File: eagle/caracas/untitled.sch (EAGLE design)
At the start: 12 parts, among them IC1 ICM7555

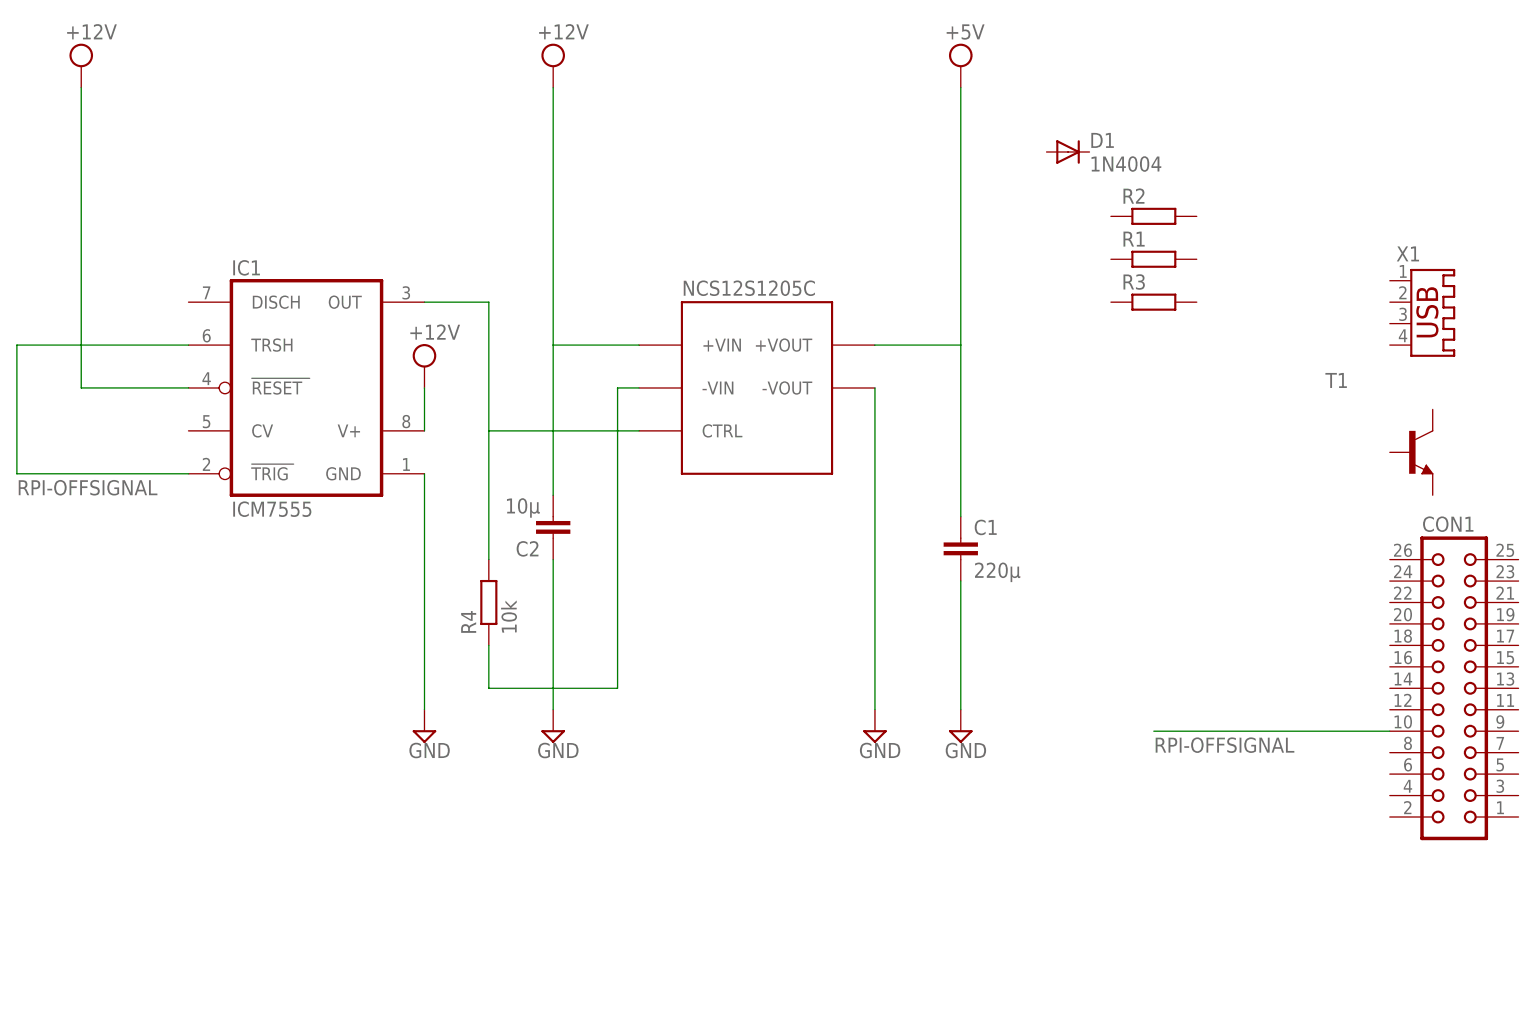
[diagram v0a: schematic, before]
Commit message: Update Eagle project.
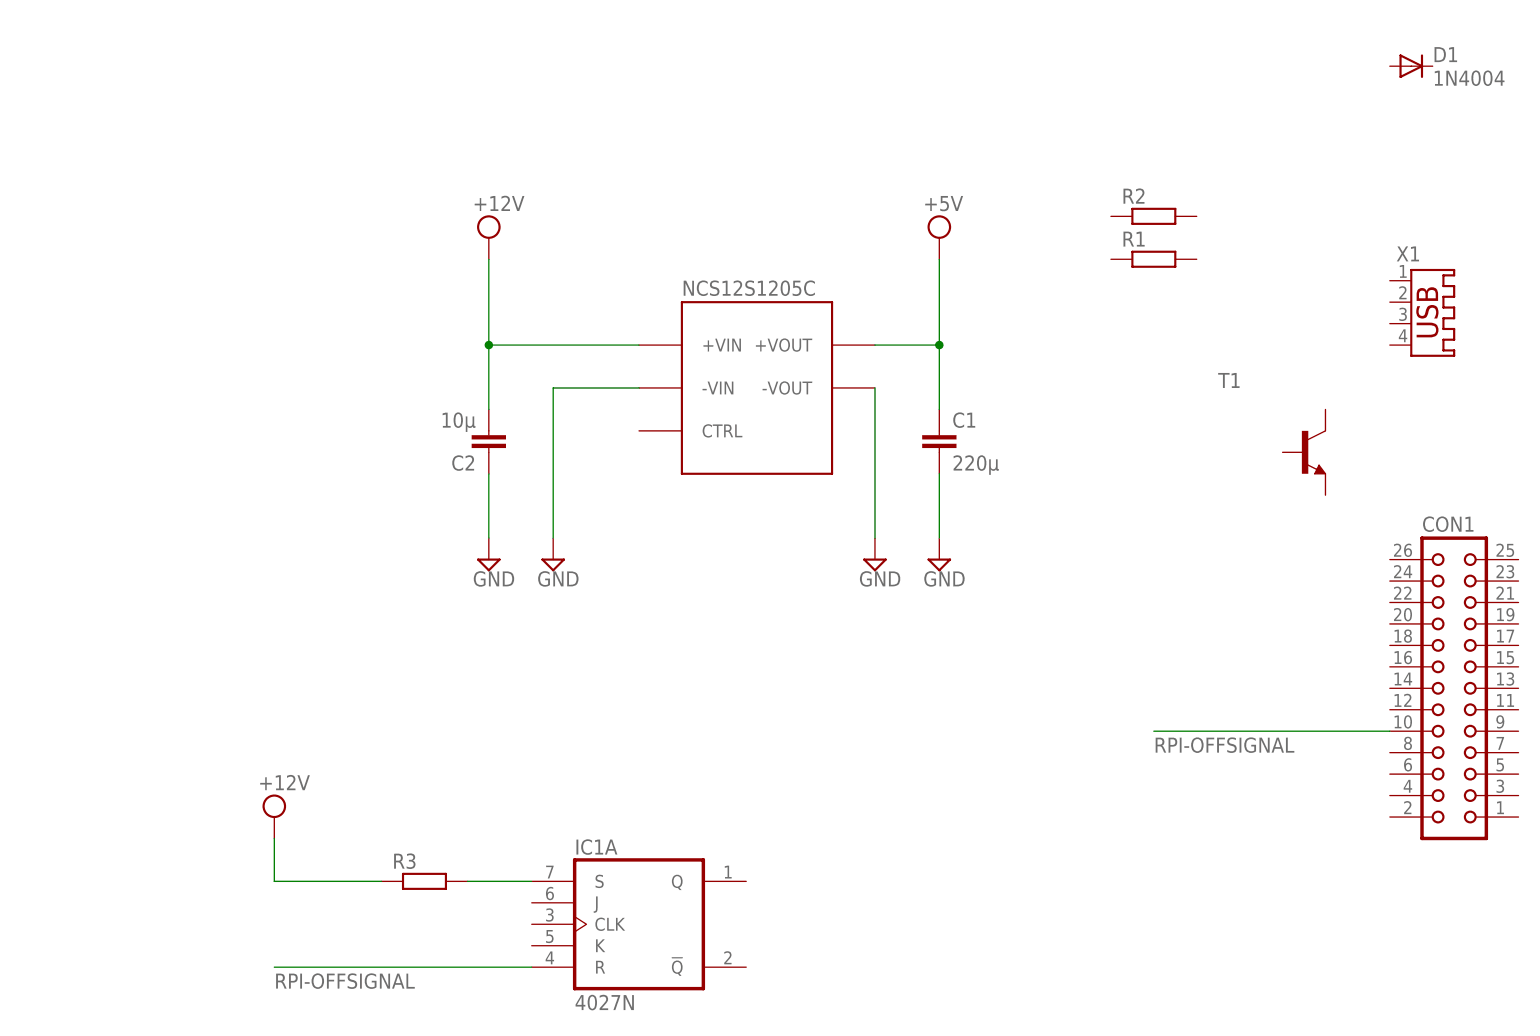
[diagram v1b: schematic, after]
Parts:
- removed R4: 10k, rcl:R-EU_0204/7
- IC1: value ICM7555 -> 4027N; device maxim:ICM7555 -> 40xx:4027N
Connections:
- removed net VCC: C1.1, C2.2, IC1.RESET, IC1.V+, U$1.+VIN, U$1.+VOUT
- new net +12V: C2.2, U$1.+VIN
- new net +12V_IGN: R3.1
- new net +5V: C1.1, U$1.+VOUT
- net GND: no longer IC1.GND, R4.1
- net N$1: now also IC1A.S, R3.2; no longer IC1.OUT, R4.2, U$1.CTRL
- net RPI-OFFSIGNAL: now also IC1A.R; no longer IC1.TRIG, IC1.TRSH
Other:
- moved on the sheet: C1, C2, D1, R3, T1
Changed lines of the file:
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@@
 <setting verticaltext="up"/>
 </settings>
-<grid distance="0.1" unitdist="inch" unit="inch" style="lines" multiple="1" display="yes" altdistance="0.01" altunitdist="inch" altunit="inch"/>
+<grid distance="0.1" unitdist="inch" unit="inch" style="lines" multiple="1" display="no" altdistance="0.01" altunitdist="inch" altunit="inch"/>
 <layers>
 <layer number="1" name="Top" color="4" fill="1" visible="no" active="no"/>
@@
 <part name="R2" library="rcl" deviceset="R-EU_" device="0207/10"/>
 <part name="R3" library="rcl" deviceset="R-EU_" device="0207/10"/>
-<part name="IC1" library="maxim" deviceset="ICM7555" device=""/>
 <part name="X1" library="con-yamaichi" deviceset="USB-A003" device=""/>
 <part name="CON1" library="con-harting" deviceset="CON26" device=""/>
@@
 <part name="D1" library="diode" deviceset="1N4004" device=""/>
 <part name="U$1" library="caracas" deviceset="NCS12S1205C" device=""/>
-<part name="R4" library="rcl" deviceset="R-EU_" device="0204/7" value="10k"/>
 <part name="SUPPLY1" library="supply2" deviceset="GND" device=""/>
 <part name="C1" library="rcl" deviceset="C-EU" device="025-024X044" value="220µ"/>
@@
 <part name="SUPPLY2" library="supply2" deviceset="GND" device=""/>
 <part name="SUPPLY3" library="supply2" deviceset="GND" device=""/>
-<part name="+12V" library="supply2" deviceset="VCC" device="" value="+12V"/>
 <part name="+5V" library="supply2" deviceset="VCC" device="" value="+5V"/>
+<part name="+12V2" library="supply2" deviceset="VCC" device="" value="+12V"/>
 <part name="SUPPLY4" library="supply2" deviceset="GND" device=""/>
-<part name="+12V1" library="supply2" deviceset="VCC" device="" value="+12V"/>
-<part name="+12V2" library="supply2" deviceset="VCC" device="" value="+12V"/>
+<part name="IC1" library="40xx" deviceset="4027" device="N"/>
+<part name="+12V_IGN" library="supply2" deviceset="VCC" device="" value="+12V"/>
 </parts>
 <sheets>
@@
 <instance part="R1" gate="G$1" x="106.68" y="73.66"/>
 <instance part="R2" gate="G$1" x="106.68" y="78.74"/>
-<instance part="R3" gate="G$1" x="106.68" y="68.58"/>
-<instance part="IC1" gate="G$1" x="7.62" y="58.42"/>
+<instance part="R3" gate="G$1" x="20.32" y="0"/>
 <instance part="X1" gate="G$1" x="139.7" y="66.04"/>
 <instance part="CON1" gate="A" x="142.24" y="22.86"/>
-<instance part="T1" gate="G$1" x="137.16" y="50.8"/>
-<instance part="D1" gate="1" x="96.52" y="86.36"/>
+<instance part="T1" gate="G$1" x="124.46" y="50.8"/>
+<instance part="D1" gate="1" x="137.16" y="96.52"/>
 <instance part="U$1" gate="G$1" x="58.42" y="58.42"/>
-<instance part="R4" gate="G$1" x="27.94" y="33.02" rot="R90"/>
-<instance part="SUPPLY1" gate="GND" x="35.56" y="17.78"/>
-<instance part="C1" gate="G$1" x="83.82" y="40.64"/>
-<instance part="C2" gate="G$1" x="35.56" y="40.64" rot="R180"/>
-<instance part="SUPPLY2" gate="GND" x="73.66" y="17.78"/>
-<instance part="SUPPLY3" gate="GND" x="83.82" y="17.78"/>
-<instance part="+12V" gate="G$1" x="-20.32" y="96.52"/>
-<instance part="+5V" gate="G$1" x="83.82" y="96.52"/>
-<instance part="SUPPLY4" gate="GND" x="20.32" y="17.78"/>
-<instance part="+12V1" gate="G$1" x="20.32" y="60.96"/>
-<instance part="+12V2" gate="G$1" x="35.56" y="96.52"/>
+<instance part="SUPPLY1" gate="GND" x="27.94" y="38.1"/>
+<instance part="C1" gate="G$1" x="81.28" y="53.34"/>
+<instance part="C2" gate="G$1" x="27.94" y="50.8" rot="R180"/>
+<instance part="SUPPLY2" gate="GND" x="73.66" y="38.1"/>
+<instance part="SUPPLY3" gate="GND" x="81.28" y="38.1"/>
+<instance part="+5V" gate="G$1" x="81.28" y="76.2"/>
+<instance part="+12V2" gate="G$1" x="27.94" y="76.2"/>
+<instance part="SUPPLY4" gate="GND" x="35.56" y="38.1"/>
+<instance part="IC1" gate="A" x="45.72" y="-5.08"/>
+<instance part="+12V_IGN" gate="G$1" x="2.54" y="7.62"/>
 </instances>
 <busses>
 </busses>
 <nets>
-<net name="N$1" class="0">
-<segment>
-<pinref part="IC1" gate="G$1" pin="OUT"/>
-<wire x1="20.32" y1="68.58" x2="27.94" y2="68.58" width="0.1524" layer="91"/>
-<wire x1="27.94" y1="68.58" x2="27.94" y2="53.34" width="0.1524" layer="91"/>
-<pinref part="U$1" gate="G$1" pin="CTRL"/>
-<wire x1="27.94" y1="53.34" x2="45.72" y2="53.34" width="0.1524" layer="91"/>
-<wire x1="27.94" y1="53.34" x2="27.94" y2="38.1" width="0.1524" layer="91"/>
-<pinref part="R4" gate="G$1" pin="2"/>
-</segment>
-</net>
 <net name="GND" class="0">
 <segment>
 <pinref part="SUPPLY1" gate="GND" pin="GND"/>
-<pinref part="R4" gate="G$1" pin="1"/>
-<wire x1="35.56" y1="20.32" x2="35.56" y2="22.86" width="0.1524" layer="91"/>
-<pinref part="U$1" gate="G$1" pin="-VIN"/>
-<wire x1="35.56" y1="22.86" x2="27.94" y2="22.86" width="0.1524" layer="91"/>
-<wire x1="27.94" y1="22.86" x2="27.94" y2="27.94" width="0.1524" layer="91"/>
-<wire x1="45.72" y1="58.42" x2="43.18" y2="58.42" width="0.1524" layer="91"/>
-<wire x1="43.18" y1="58.42" x2="43.18" y2="22.86" width="0.1524" layer="91"/>
-<wire x1="43.18" y1="22.86" x2="35.56" y2="22.86" width="0.1524" layer="91"/>
 <pinref part="C2" gate="G$1" pin="1"/>
-<wire x1="35.56" y1="38.1" x2="35.56" y2="22.86" width="0.1524" layer="91"/>
+<wire x1="27.94" y1="48.26" x2="27.94" y2="40.64" width="0.1524" layer="91"/>
 </segment>
 <segment>
 <pinref part="U$1" gate="G$1" pin="-VOUT"/>
-<wire x1="73.66" y1="58.42" x2="73.66" y2="20.32" width="0.1524" layer="91"/>
+<wire x1="73.66" y1="58.42" x2="73.66" y2="40.64" width="0.1524" layer="91"/>
 <pinref part="SUPPLY2" gate="GND" pin="GND"/>
 </segment>
@@
 <pinref part="C1" gate="G$1" pin="2"/>
 <pinref part="SUPPLY3" gate="GND" pin="GND"/>
-<wire x1="83.82" y1="35.56" x2="83.82" y2="20.32" width="0.1524" layer="91"/>
+<wire x1="81.28" y1="48.26" x2="81.28" y2="40.64" width="0.1524" layer="91"/>
 </segment>
 <segment>
-<pinref part="IC1" gate="G$1" pin="GND"/>
-<wire x1="20.32" y1="48.26" x2="20.32" y2="20.32" width="0.1524" layer="91"/>
+<pinref part="U$1" gate="G$1" pin="-VIN"/>
+<wire x1="45.72" y1="58.42" x2="35.56" y2="58.42" width="0.1524" layer="91"/>
 <pinref part="SUPPLY4" gate="GND" pin="GND"/>
+<wire x1="35.56" y1="40.64" x2="35.56" y2="58.42" width="0.1524" layer="91"/>
 </segment>
 </net>
-<net name="VCC" class="0">
-<segment>
-<pinref part="+12V" gate="G$1" pin="VCC"/>
-<pinref part="IC1" gate="G$1" pin="RESET"/>
-<wire x1="-7.62" y1="58.42" x2="-20.32" y2="58.42" width="0.1524" layer="91"/>
-<wire x1="-20.32" y1="58.42" x2="-20.32" y2="93.98" width="0.1524" layer="91"/>
-</segment>
+<net name="+5V" class="0">
 <segment>
 <pinref part="C1" gate="G$1" pin="1"/>
-<wire x1="83.82" y1="43.18" x2="83.82" y2="63.5" width="0.1524" layer="91"/>
+<wire x1="81.28" y1="55.88" x2="81.28" y2="63.5" width="0.1524" layer="91"/>
 <pinref part="U$1" gate="G$1" pin="+VOUT"/>
-<wire x1="83.82" y1="63.5" x2="73.66" y2="63.5" width="0.1524" layer="91"/>
+<wire x1="81.28" y1="63.5" x2="73.66" y2="63.5" width="0.1524" layer="91"/>
 <pinref part="+5V" gate="G$1" pin="VCC"/>
-<wire x1="83.82" y1="93.98" x2="83.82" y2="63.5" width="0.1524" layer="91"/>
-</segment>
-<segment>
-<pinref part="IC1" gate="G$1" pin="V+"/>
-<pinref part="+12V1" gate="G$1" pin="VCC"/>
-<wire x1="20.32" y1="53.34" x2="20.32" y2="58.42" width="0.1524" layer="91"/>
-</segment>
-<segment>
-<pinref part="C2" gate="G$1" pin="2"/>
-<wire x1="35.56" y1="45.72" x2="35.56" y2="63.5" width="0.1524" layer="91"/>
-<pinref part="U$1" gate="G$1" pin="+VIN"/>
-<wire x1="35.56" y1="63.5" x2="45.72" y2="63.5" width="0.1524" layer="91"/>
-<pinref part="+12V2" gate="G$1" pin="VCC"/>
-<wire x1="35.56" y1="63.5" x2="35.56" y2="93.98" width="0.1524" layer="91"/>
+<wire x1="81.28" y1="73.66" x2="81.28" y2="63.5" width="0.1524" layer="91"/>
+<junction x="81.28" y="63.5"/>
 </segment>
 </net>
@@
 </segment>
 <segment>
-<pinref part="IC1" gate="G$1" pin="TRIG"/>
-<wire x1="-7.62" y1="48.26" x2="-27.94" y2="48.26" width="0.1524" layer="91"/>
-<label x="-27.94" y="45.72" size="1.778" layer="95"/>
-<pinref part="IC1" gate="G$1" pin="TRSH"/>
-<wire x1="-7.62" y1="63.5" x2="-27.94" y2="63.5" width="0.1524" layer="91"/>
-<wire x1="-27.94" y1="63.5" x2="-27.94" y2="48.26" width="0.1524" layer="91"/>
+<pinref part="IC1" gate="A" pin="R"/>
+<wire x1="33.02" y1="-10.16" x2="2.54" y2="-10.16" width="0.1524" layer="91"/>
+<label x="2.54" y="-12.7" size="1.778" layer="95"/>
 </segment>
 </net>
+<net name="N$1" class="0">
+<segment>
+<pinref part="R3" gate="G$1" pin="2"/>
+<pinref part="IC1" gate="A" pin="S"/>
+<wire x1="25.4" y1="0" x2="33.02" y2="0" width="0.1524" layer="91"/>
+</segment>
+</net>
+<net name="+12V_IGN" class="0">
+<segment>
+<pinref part="R3" gate="G$1" pin="1"/>
+<wire x1="15.24" y1="0" x2="2.54" y2="0" width="0.1524" layer="91"/>
+<wire x1="2.54" y1="0" x2="2.54" y2="5.08" width="0.1524" layer="91"/>
+<pinref part="+12V_IGN" gate="G$1" pin="VCC"/>
+</segment>
+</net>
+<net name="+12V" class="0">
+<segment>
+<pinref part="C2" gate="G$1" pin="2"/>
+<wire x1="27.94" y1="55.88" x2="27.94" y2="63.5" width="0.1524" layer="91"/>
+<pinref part="U$1" gate="G$1" pin="+VIN"/>
+<wire x1="27.94" y1="63.5" x2="45.72" y2="63.5" width="0.1524" layer="91"/>
+<pinref part="+12V2" gate="G$1" pin="VCC"/>
+<wire x1="27.94" y1="63.5" x2="27.94" y2="73.66" width="0.1524" layer="91"/>
+<junction x="27.94" y="63.5"/>
+</segment>
+</net>
